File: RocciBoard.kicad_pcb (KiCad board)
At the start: 2 copper layers, 99 x 54 mm, 195 parts, among them J1 Battery, J10 M3, J11 I2C6, J12 Power, J13 M2, J14 I2C7, J2 I2C0, J3 I2C1, J4 I2C2, J5 I2C3, J6 M0, J7 I2C4, J8 M1, J9 I2C5, Q1 IRF7404, Q2 2N7002, U1 LMR33630, U10 LM317_TO-252, U2 LM317_TO-252, U3 LM317_TO-252, U4 TPS3700, U5 TCA9548A, U6 DRV8871, U7 DRV8871, U8 DRV8871, U9 DRV8871

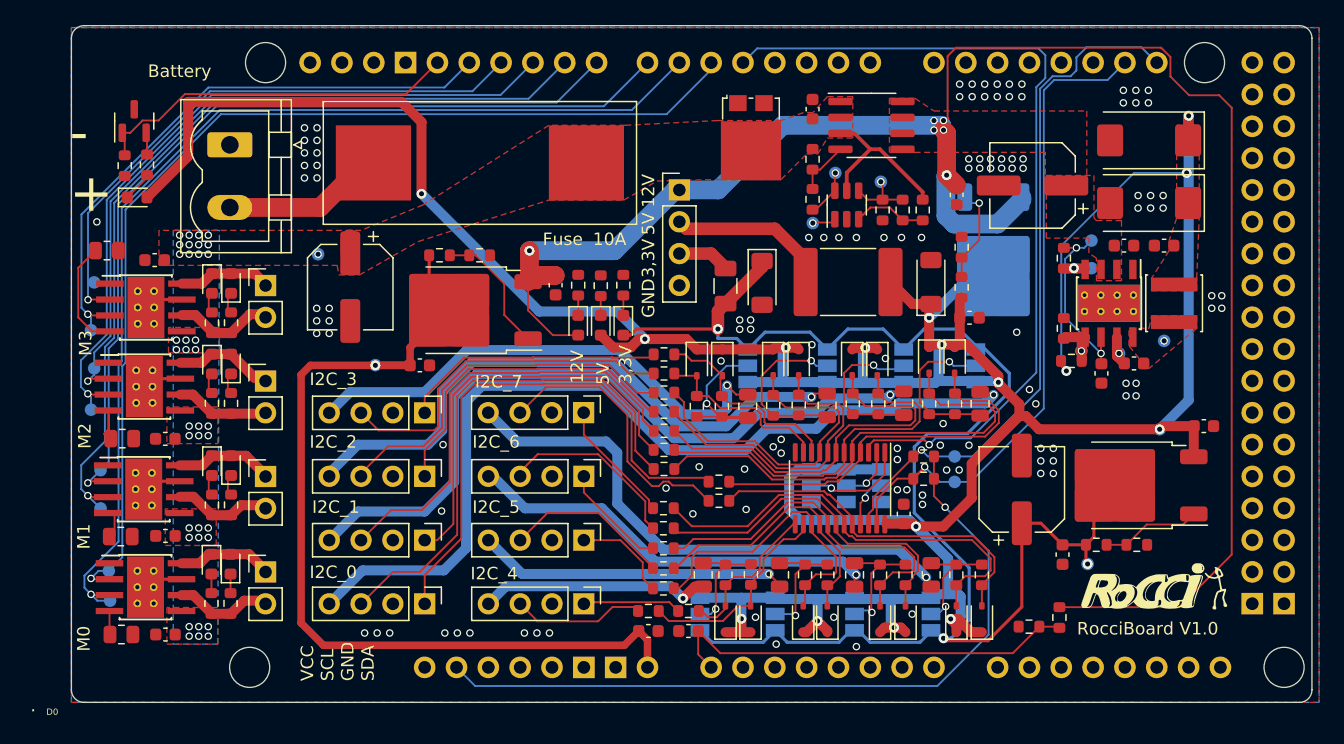
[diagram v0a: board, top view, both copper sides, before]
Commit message: final version V1.0
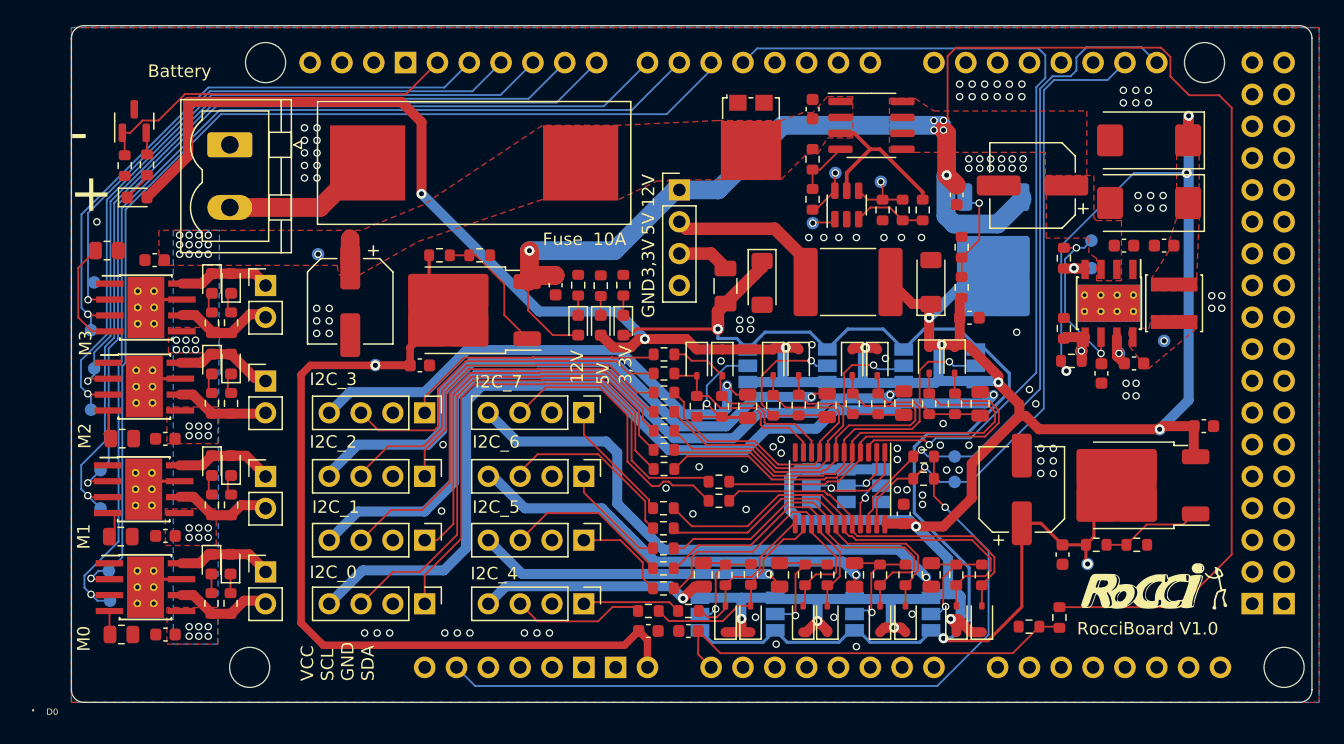
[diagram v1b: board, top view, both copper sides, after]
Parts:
- moved U2 2.08 mm to (206.2, 114.0)
- moved U3 1.87 mm to (152.9, 100.0)
- moved C14 1.13 mm to (141.9, 99.3)
- moved D32 0.68 mm to (173.9, 85.6)
- moved F2 0.46 mm to (151.8, 88.3)
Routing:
- net +12V: track 14.4 -> 15.5 mm
